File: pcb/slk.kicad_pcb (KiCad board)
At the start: 2 copper layers, 68.6 x 53.3 mm, 22 parts, among them J1 Screw Terminal, P1 Power, P2 Analog, P3 Digital 1, P4 Digital 2, SW1 SW_SPDT, U1 MCP2515-xSO, U2 TJA1055T1, Y1 16MHz

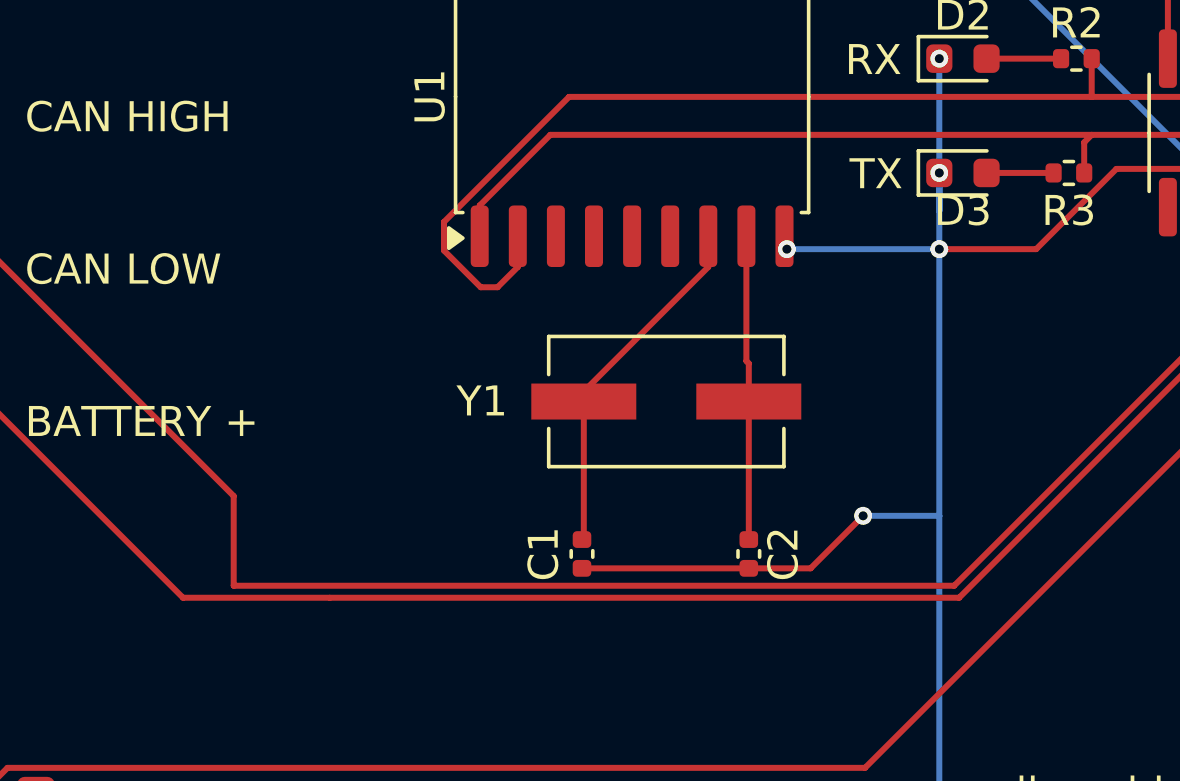
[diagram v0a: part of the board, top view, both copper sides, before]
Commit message: done
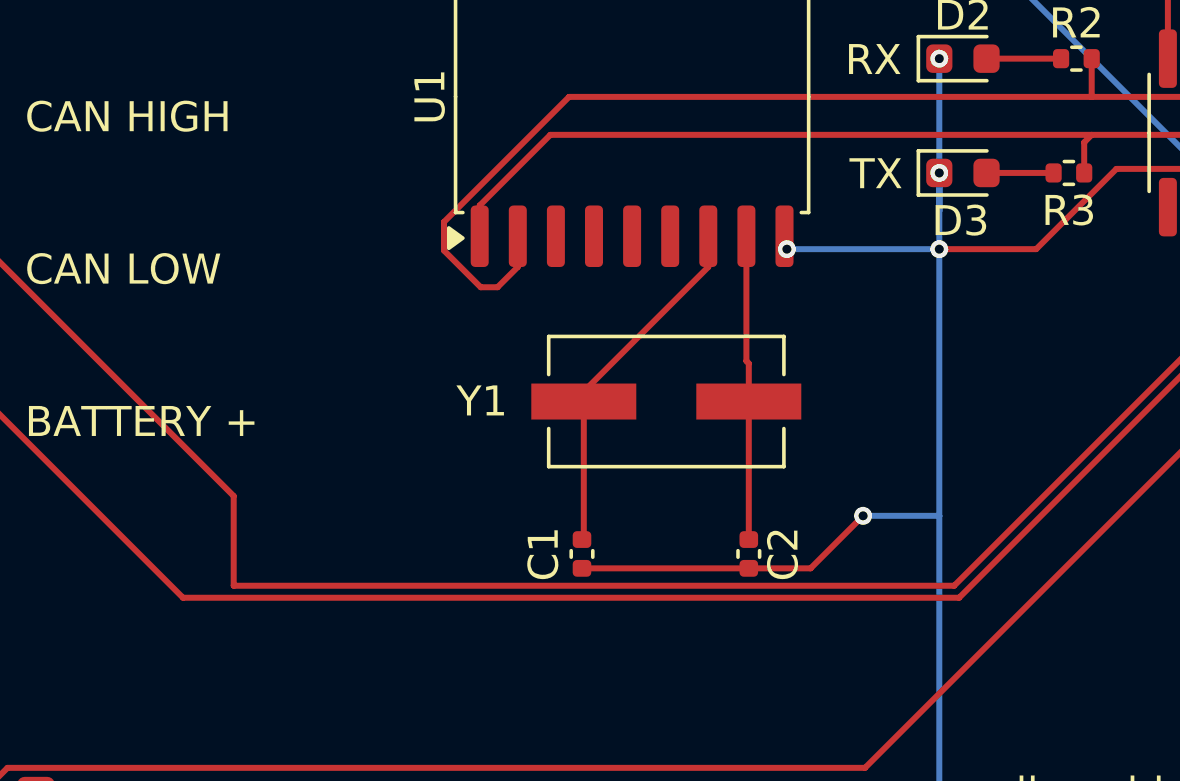
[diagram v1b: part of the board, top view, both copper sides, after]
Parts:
- R1, R2, R3: value R -> 330
